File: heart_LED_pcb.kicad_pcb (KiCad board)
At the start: 4 copper layers, 85.8 x 78.4 mm, 73 parts, among them J1 USB_C_2.0_16P, SW1 EN, SW2 BOOT, SW3 MODE, SW4 LED_MODUS, U1 ESP32-C3, U2 AMS1117-3.3, Y1 40 MHz

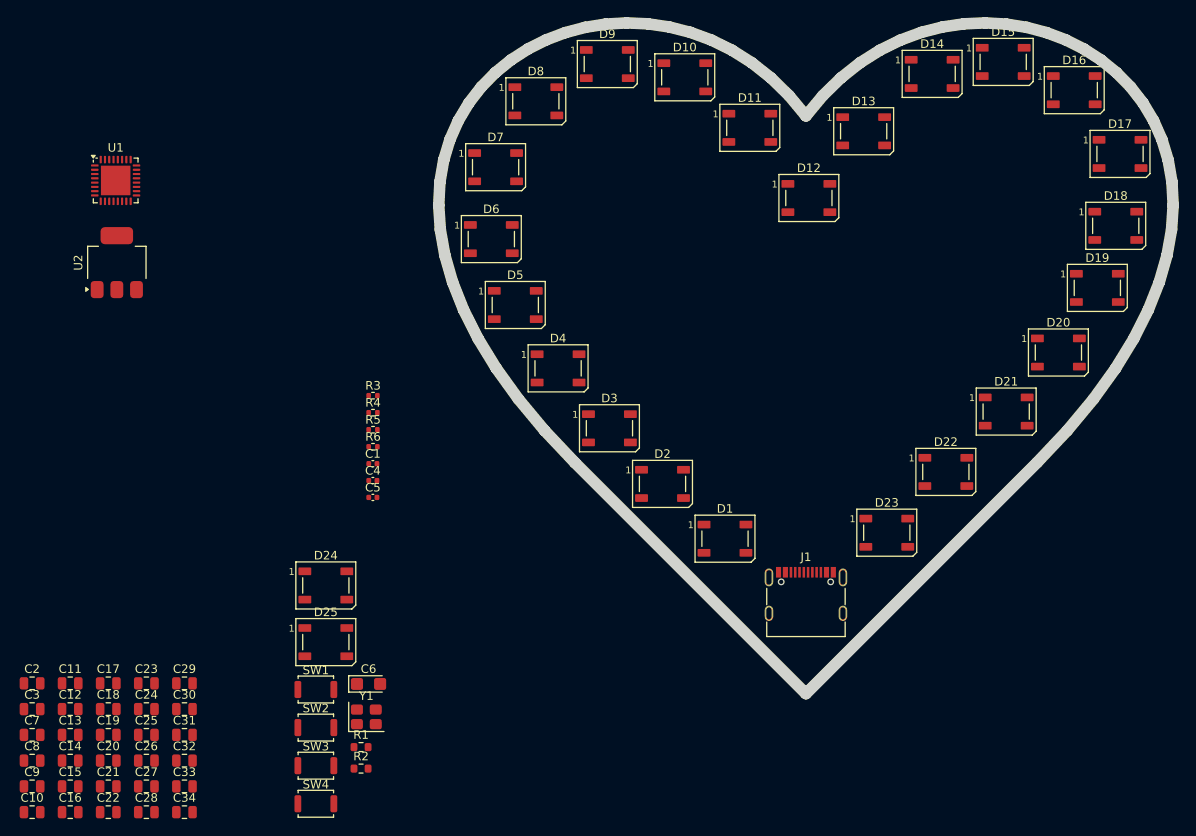
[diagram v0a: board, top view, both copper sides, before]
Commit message: Updated schematic
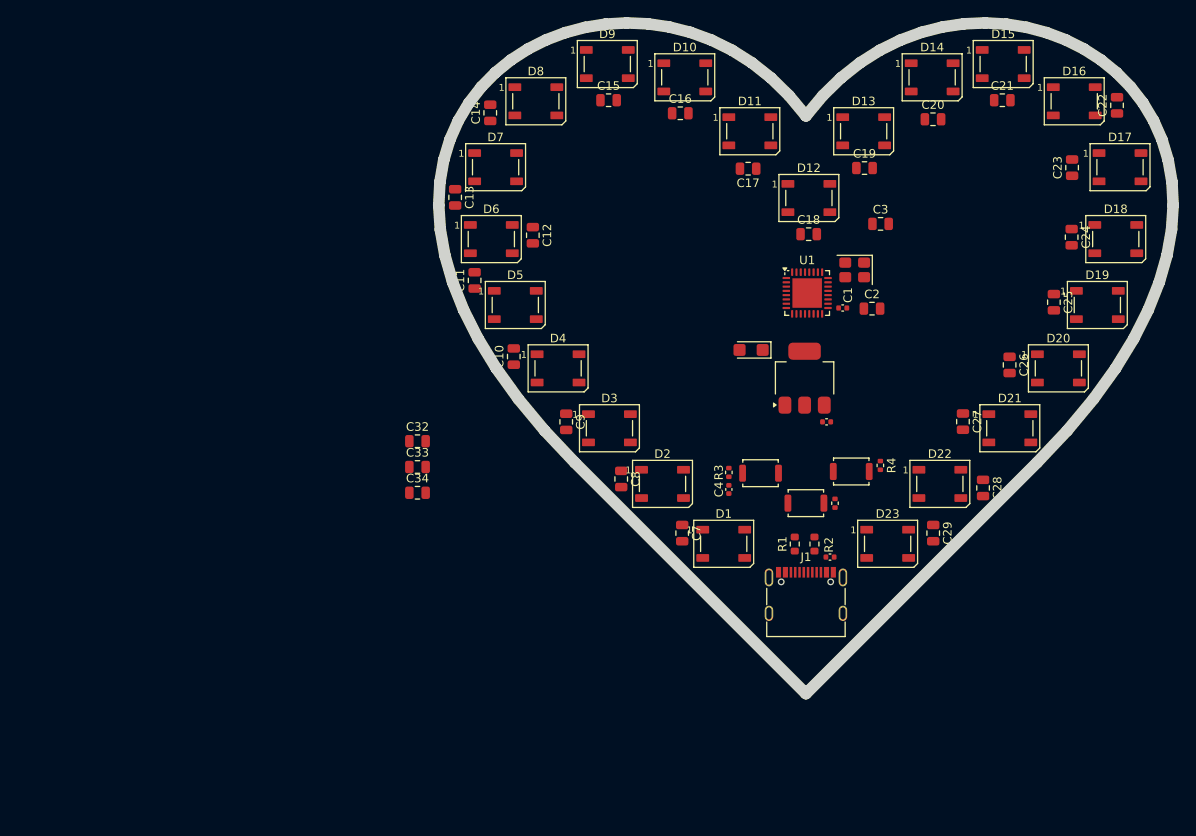
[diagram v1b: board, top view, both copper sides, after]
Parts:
- removed C30, C31: 100nF, Capacitor_SMD:C_0805_2012Metric
- removed D24, D25: WS2812B, LED_SMD:LED_WS2812B_PLCC4_5.0x5.0mm_P3.2mm
- removed R5: 10k, Resistor_SMD:R_0402_1005Metric
- removed the SW3 at (93.8, 148.6)
- added C35: 100nF, Capacitor_SMD:C_0402_1005Metric, F.Cu at (153.9, 124.2)
- moved C22 143.9 mm to (187.4, 71.4), turned to 90 degrees
- moved C21 131.7 mm to (174.1, 70.8)
- moved C23 123.8 mm to (182.2, 78.7), turned to 90 degrees
- moved C20 122.1 mm to (165.9, 73.0)
- moved C24 121.3 mm to (182.2, 86.8), turned to -90 degrees
- moved C25 117.5 mm to (180.1, 94.4), turned to -90 degrees
- moved C3 114.2 mm to (159.8, 85.3)
- moved C26 110.9 mm to (174.9, 101.8), turned to -90 degrees
- moved C19 110.4 mm to (157.9, 78.8)
- moved C16 108.4 mm to (136.4, 72.3)
- moved C2 107.4 mm to (158.8, 95.2)
- moved C28 104.8 mm to (171.8, 116.1), turned to -90 degrees
- moved C27 104.5 mm to (169.4, 108.4), turned to -90 degrees
- moved C15 101.9 mm to (128.1, 70.8)
- moved C18 98.9 mm to (151.4, 86.5)
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- renumbered SW4 to SW3
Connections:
- D23 pad 2: Net-(D23-DOUT) -> unconnected-(D23-DOUT-Pad2)
- U1 pad 14: /LED_MODUS -> unconnected-(U1-GPIO8-Pad14)
- U1 pad 16: /LED_PWM -> /LED_MODUS
